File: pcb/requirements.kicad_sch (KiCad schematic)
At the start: 13 parts

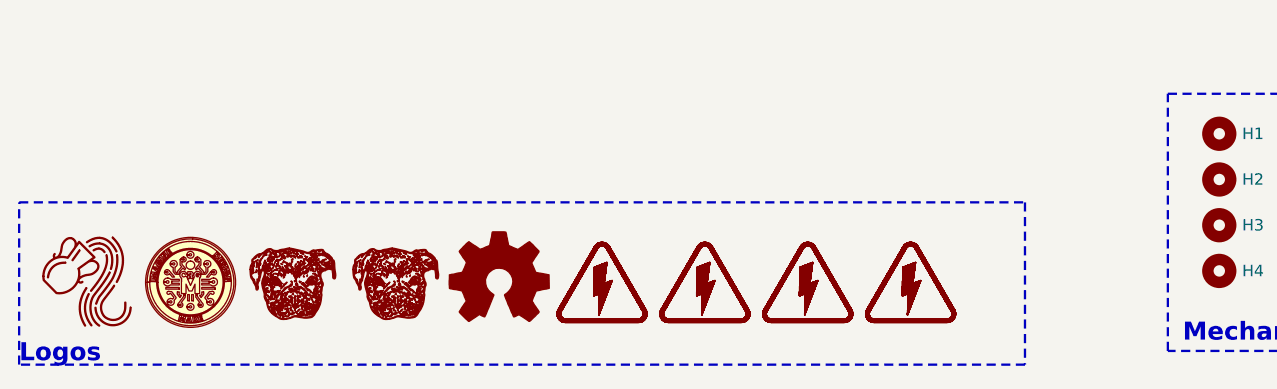
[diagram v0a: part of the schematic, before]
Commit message: Clean up, arranging, ERC and DCR
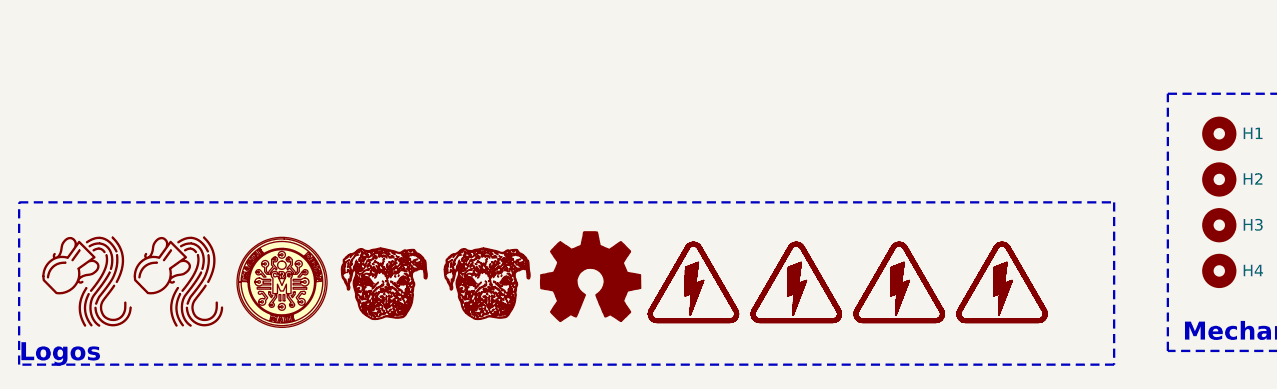
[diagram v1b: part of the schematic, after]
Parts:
- added LOGO6: ~, CRGM Logos:Aquarius Logo 5mm, symbol CRGM Logos:Aquarius Logo
- LOGO2: footprint CRGM Logos:Roxy 5mm -> CRGM Logos:Roxy 3.5mm
